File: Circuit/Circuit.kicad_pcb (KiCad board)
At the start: 2 copper layers, 62.6 x 59.3 mm, 14 parts, among them J1 Conn_01x20, J2 Conn_01x20, U1 TL072, U2 AMS1117-3.3, Y1 Crystal

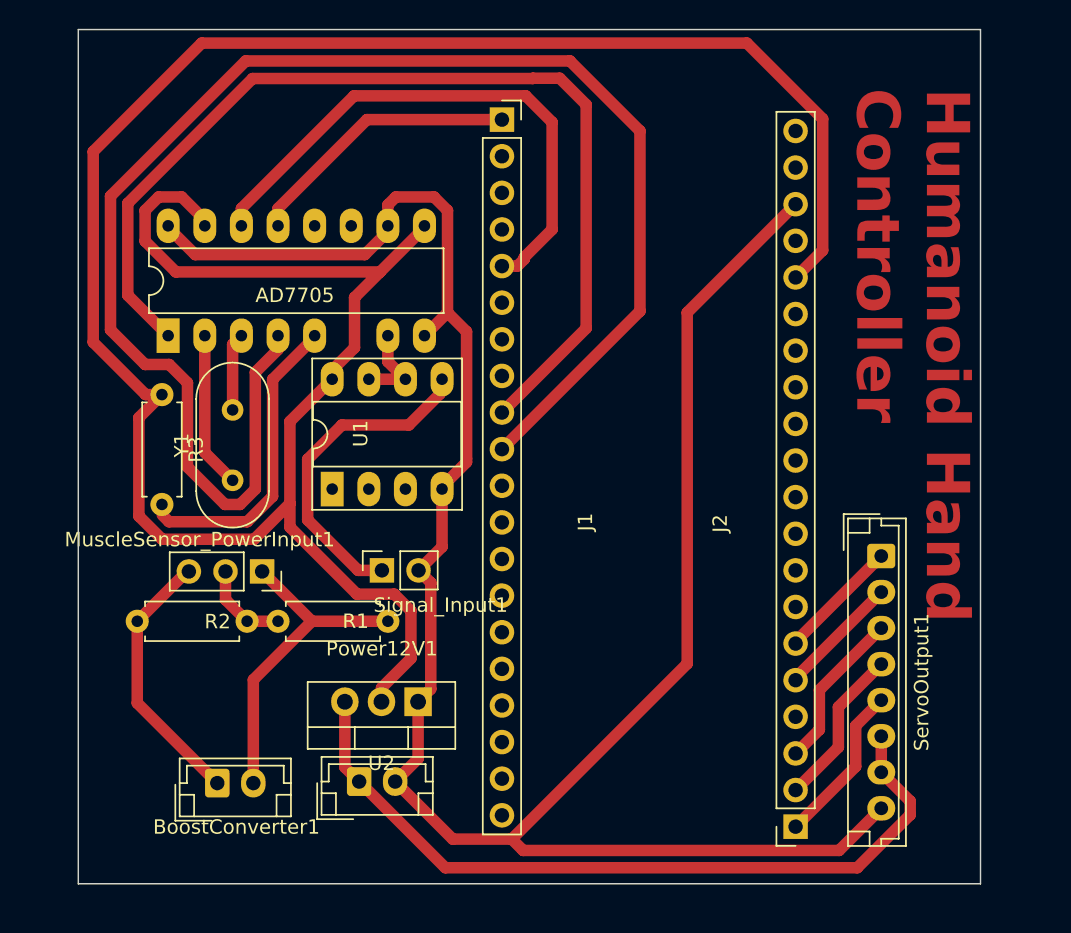
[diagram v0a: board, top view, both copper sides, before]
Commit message: final PCB design done
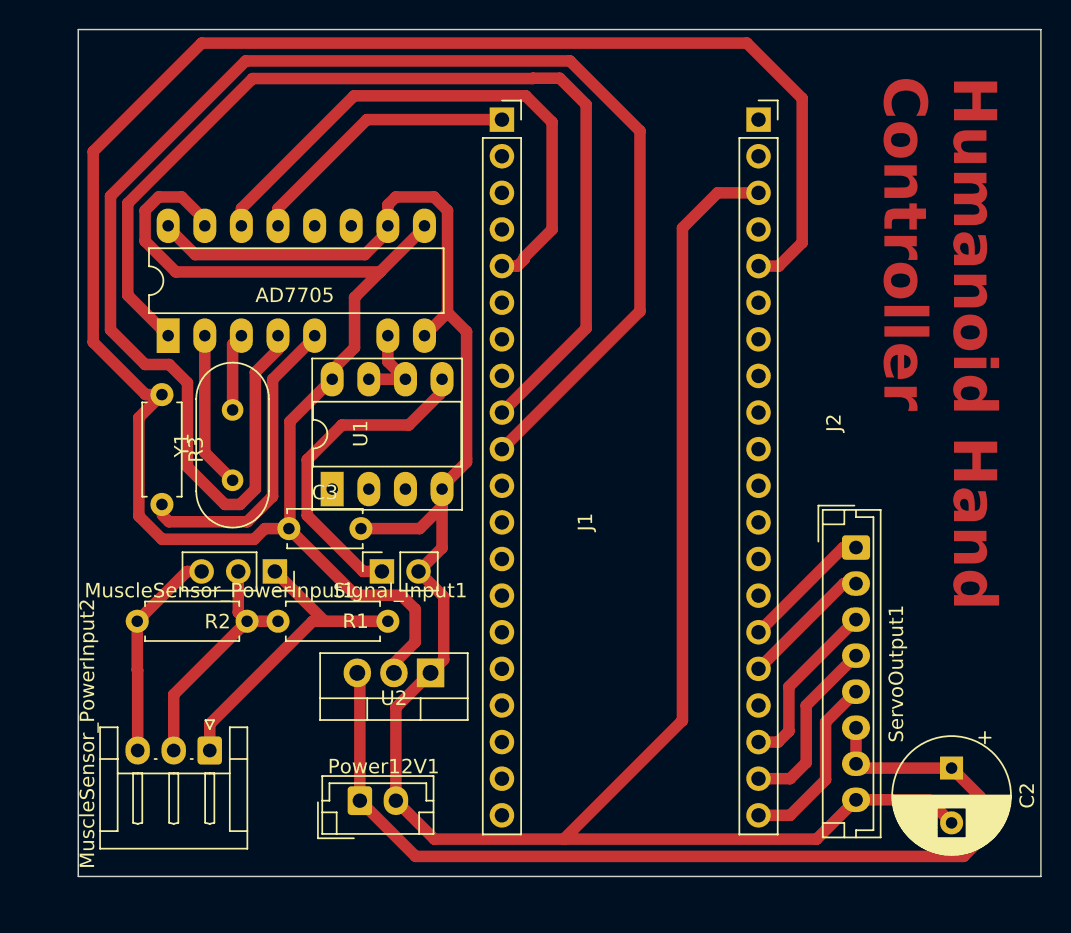
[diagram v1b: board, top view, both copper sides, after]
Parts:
- removed BoostConverter1: Conn_01x02, Connector_JST:JST_EH_B2B-EH-A_1x02_P2.50mm_Vertical
- added C2: 330uF, Capacitor_THT:CP_Radial_D8.0mm_P3.80mm, F.Cu at (147.5, 121.3)
- added C3: 10nF, Capacitor_THT:C_Disc_D5.0mm_W2.5mm_P5.00mm, F.Cu at (101.5, 104.6)
- added MuscleSensor_PowerInput2: Conn_01x03, Connector_JST:JST_EH_S3B-EH_1x03_P2.50mm_Horizontal, F.Cu at (96.0, 120.0)
- moved J2 49.1 mm to (134.1, 76.3), turned to 0 degrees
- moved U2 2.18 mm to (111.4, 114.7)
- moved ServoOutput1 1.85 mm to (140.9, 106.0)
- moved Power12V1 1.33 mm to (106.5, 123.5)
- moved MuscleSensor_PowerInput1 0.89 mm to (100.6, 107.6)
- moved Signal_Input1 0.08 mm to (108.0, 107.6)
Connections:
- J2 pad 1: Servo5 -> unconnected-(J2-Pin_1-Pad1)
- J2 pad 15: unconnected-(J2-Pin_15-Pad15) -> Servo1
- J2 pad 16: +3.3V -> Servo2
- J2 pad 18: GND -> Servo3
- J2 pad 19: unconnected-(J2-Pin_19-Pad19) -> Servo4
- J2 pad 2: Servo4 -> unconnected-(J2-Pin_2-Pad2)
- J2 pad 20: unconnected-(J2-Pin_20-Pad20) -> Servo5
- J2 pad 3: Servo3 -> GND
- J2 pad 5: Servo2 -> +3.3V
- J2 pad 6: Servo1 -> unconnected-(J2-Pin_6-Pad6)
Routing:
- net +12V: track 54.5 -> 69.1 mm
- net GND: track 157.8 -> 171.7 mm
- net Net-(MuscleSensor_PowerInput1-Pin_2): track 6.22 -> 16.9 mm
- net +24V: track 18.5 -> 14.9 mm
- net +3.3V: track 176.1 -> 173.5 mm
- net Servo4: track 11.2 -> 12.6 mm
- net Servo5: track 11.2 -> 12.7 mm
- net GNDA: track 23.1 -> 22.0 mm
- net Servo3: track 11.2 -> 12.1 mm
- net Servo1: track 8.54 -> 9.20 mm
- net Servo2: track 8.58 -> 9.21 mm
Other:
- board size 62.6 x 59.3 mm -> 66.8 x 58.8 mm
